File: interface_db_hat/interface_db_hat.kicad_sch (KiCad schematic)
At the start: 56 parts, among them J2 Conn_02x06_Counter_Clockwise, J3 Conn_02x06_Counter_Clockwise, J6 Conn_01x04_Pin, J7 Conn_01x20_Pin, Q1 BC817

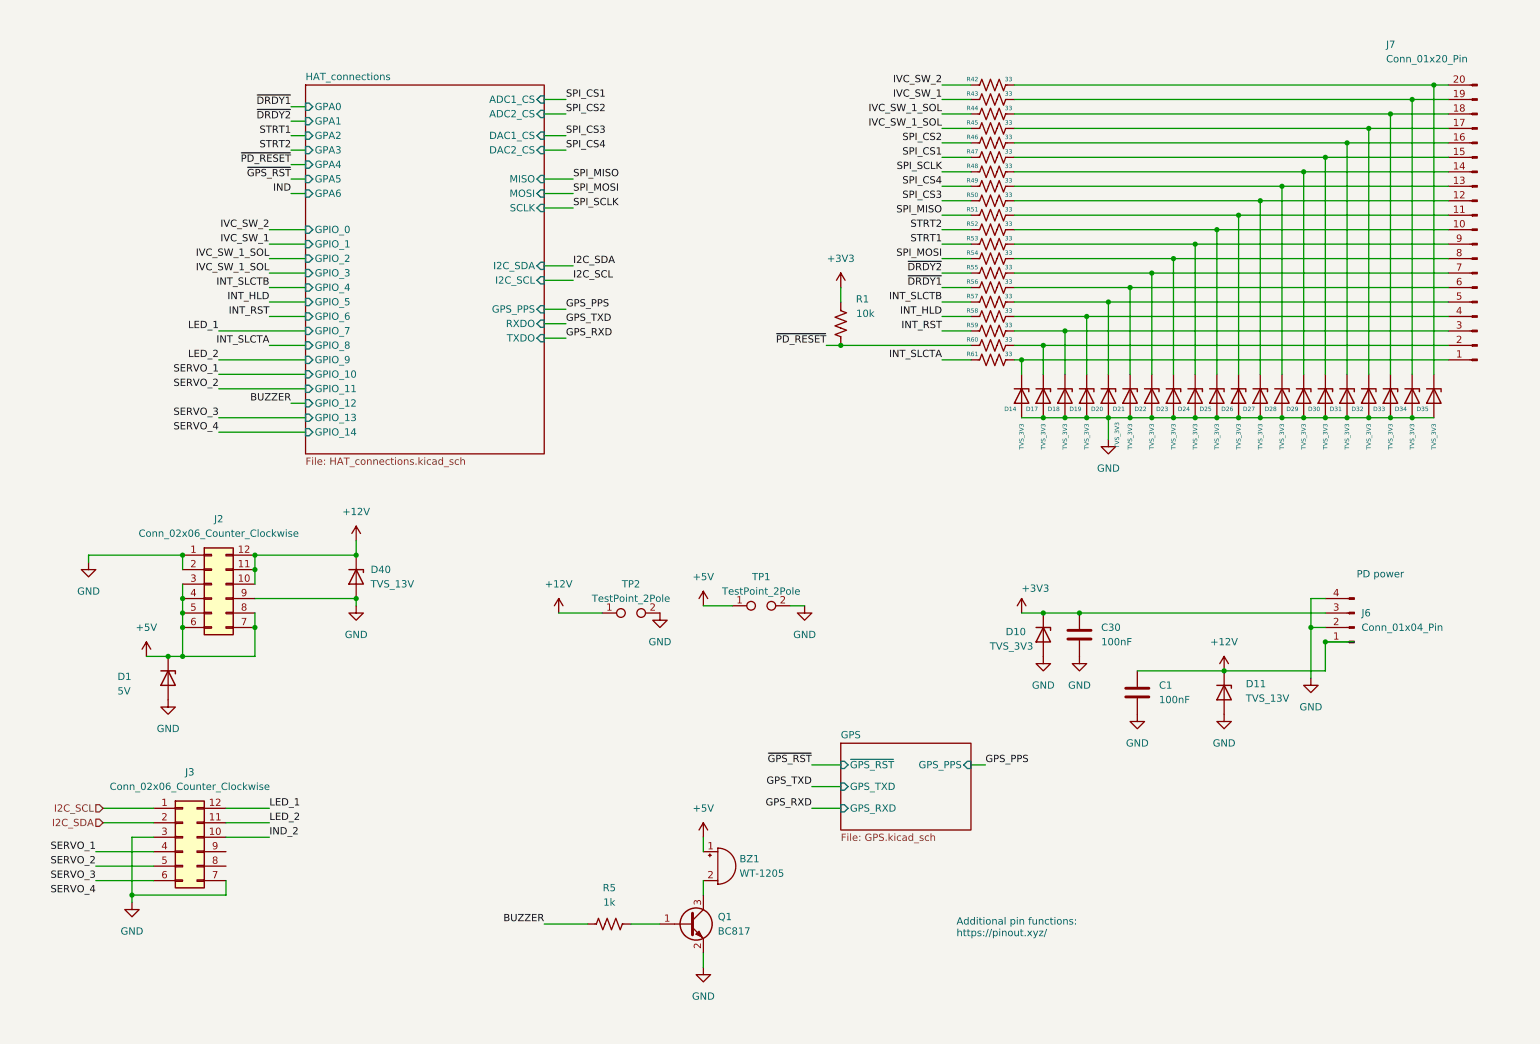
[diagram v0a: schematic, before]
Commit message: UPDATE
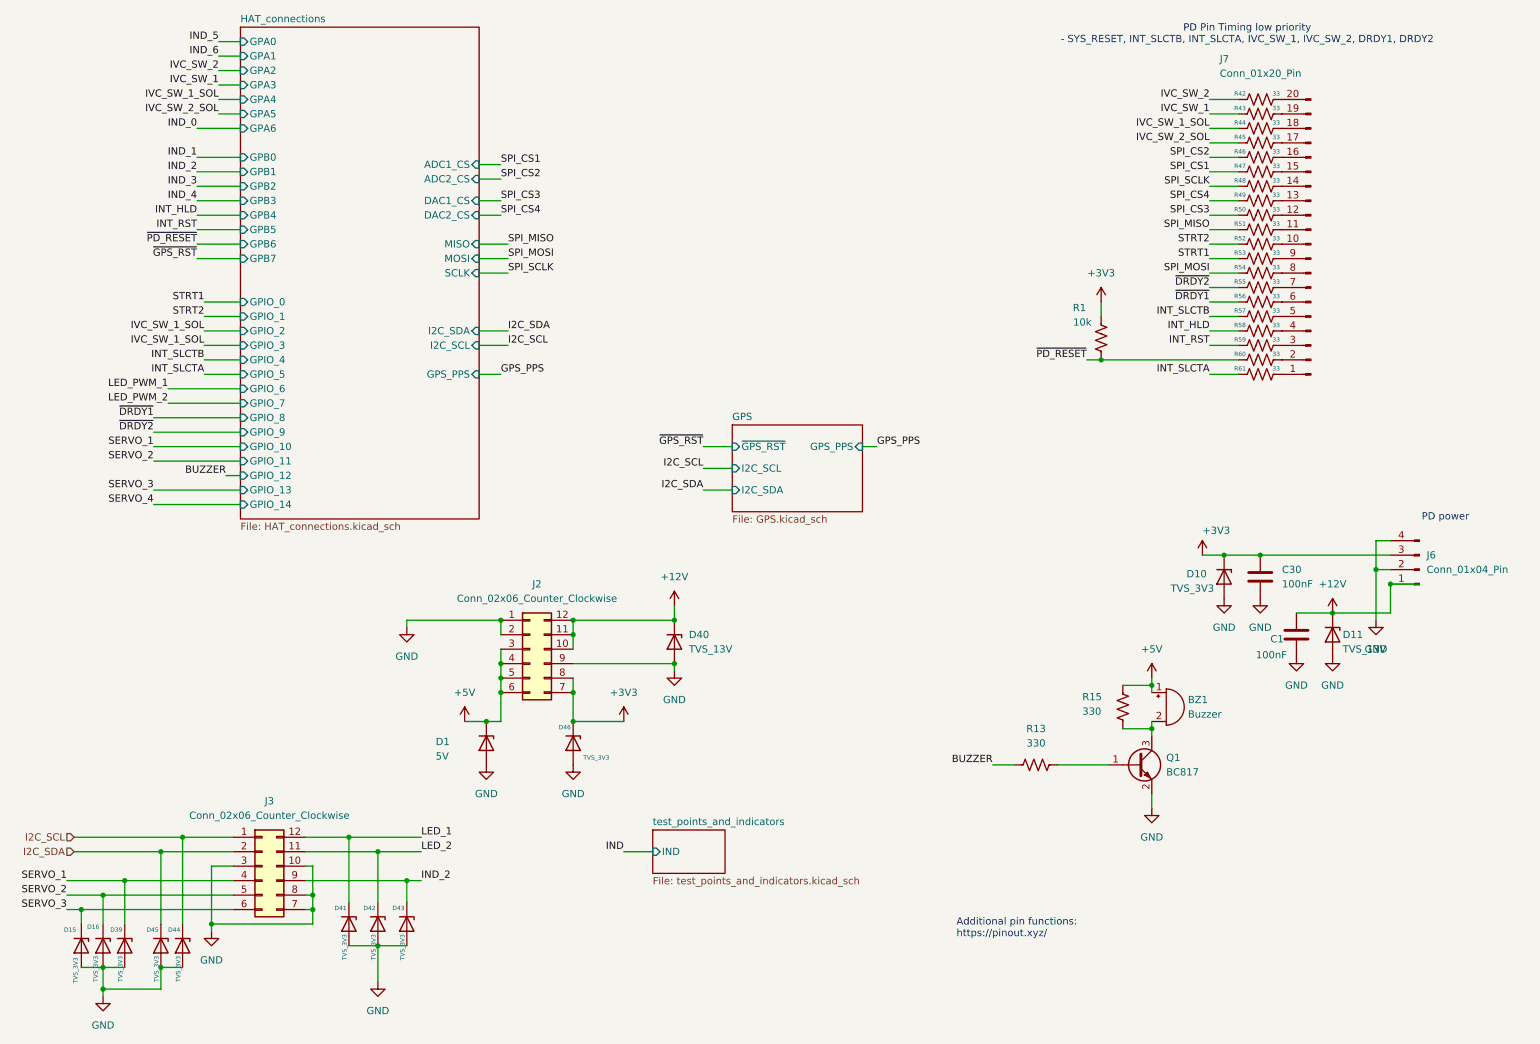
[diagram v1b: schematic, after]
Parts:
- removed D14, D17, D18, D19, D20, D21, D22, D23, D24, D25, D26, D27, D28, D29, D30, D31, D32, D33, D34, D35: TVS_3V3, Diode_SMD:D_0603_1608Metric_Pad1.05x0.95mm_HandSolder, symbol Device:D_Zener
- removed R5: 1k, symbol Device:R_US
- removed TP1, TP2: TestPoint_2Pole, Connector_PinHeader_2.54mm:PinHeader_1x02_P2.54mm_Vertical, symbol Connector:TestPoint_2Pole
- added D15, D16, D39, D41, D42, D43, D44, D45, D46: TVS_3V3, Diode_SMD:D_0402_1005Metric_Pad0.77x0.64mm_HandSolder, symbol Device:D_Zener
- added R13, R15: 330, Resistor_SMD:R_0603_1608Metric_Pad0.98x0.95mm_HandSolder, symbol Device:R_US
- BZ1: value WT-1205 -> Buzzer; footprint (none) -> Buzzer_Beeper:Buzzer_12x9.5RM7.6
- D10: footprint Diode_SMD:D_0603_1608Metric_Pad1.05x0.95mm_HandSolder -> Diode_SMD:D_0402_1005Metric_Pad0.77x0.64mm_HandSolder
- R1: footprint (none) -> Resistor_SMD:R_0603_1608Metric_Pad0.98x0.95mm_HandSolder
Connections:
- net +3V3: now also J2.7 (Pin_7), J2.8 (Pin_8), D46.1 (K)
- net +5V: now also R15.1; no longer J2.7 (Pin_7), J2.8 (Pin_8)
- net BUZZER: now also R13.1
- net GND: now also J3.10 (Pin_10), J3.8 (Pin_8), D15.2 (A), D16.2 (A), D39.2 (A), D41.2 (A), D42.2 (A), D43.2 (A), D44.2 (A), D45.2 (A), D46.2 (A)
- net I2C_SCL: now also D44.1 (K)
- net I2C_SDA: now also D45.1 (K)
- net IND_2: now also J3.9 (Pin_9), D43.1 (K); no longer J3.10 (Pin_10)
- net IVC_SW_1_SOL: no longer R45.1
- net LED_1: now also D41.1 (K)
- net LED_2: now also D42.1 (K)
- net SERVO_1: now also D39.1 (K)
- net SERVO_2: now also D16.1 (K)
- net SERVO_3: now also D15.1 (K)
- net at BZ1.2 (-), Q1.3 (C): now also R15.2
- net at Q1.1 (B): now also R13.2
- new net IVC_SW_2_SOL: R45.1
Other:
- added sheet test_points_and_indicators (test_points_and_indicators.kicad_sch)
- sheet GPS ports: added I2C_SCL, I2C_SDA; removed GPS_RXD, GPS_TXD
- sheet HAT_connections ports: added GPB0, GPB1, GPB2, GPB3, GPB4, GPB5, GPB6, GPB7; removed RXDO, TXDO
- note added: "PD Pin Timing low priority - SYS_RESET, INT_SLCTB, INT_SLCTA, IVC_SW_1, IVC_SW_2, DRDY1, DRDY2"
- moved on the sheet: BZ1, C1, C30, D1, D10, D11, D40, J2, J3, J6, J7, Q1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
